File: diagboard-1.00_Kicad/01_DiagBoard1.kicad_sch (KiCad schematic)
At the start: 34 parts, among them IC1 27C512, IC2 7400N, IC3 74273N, IC4 7404N, Q1 1.000 MHz

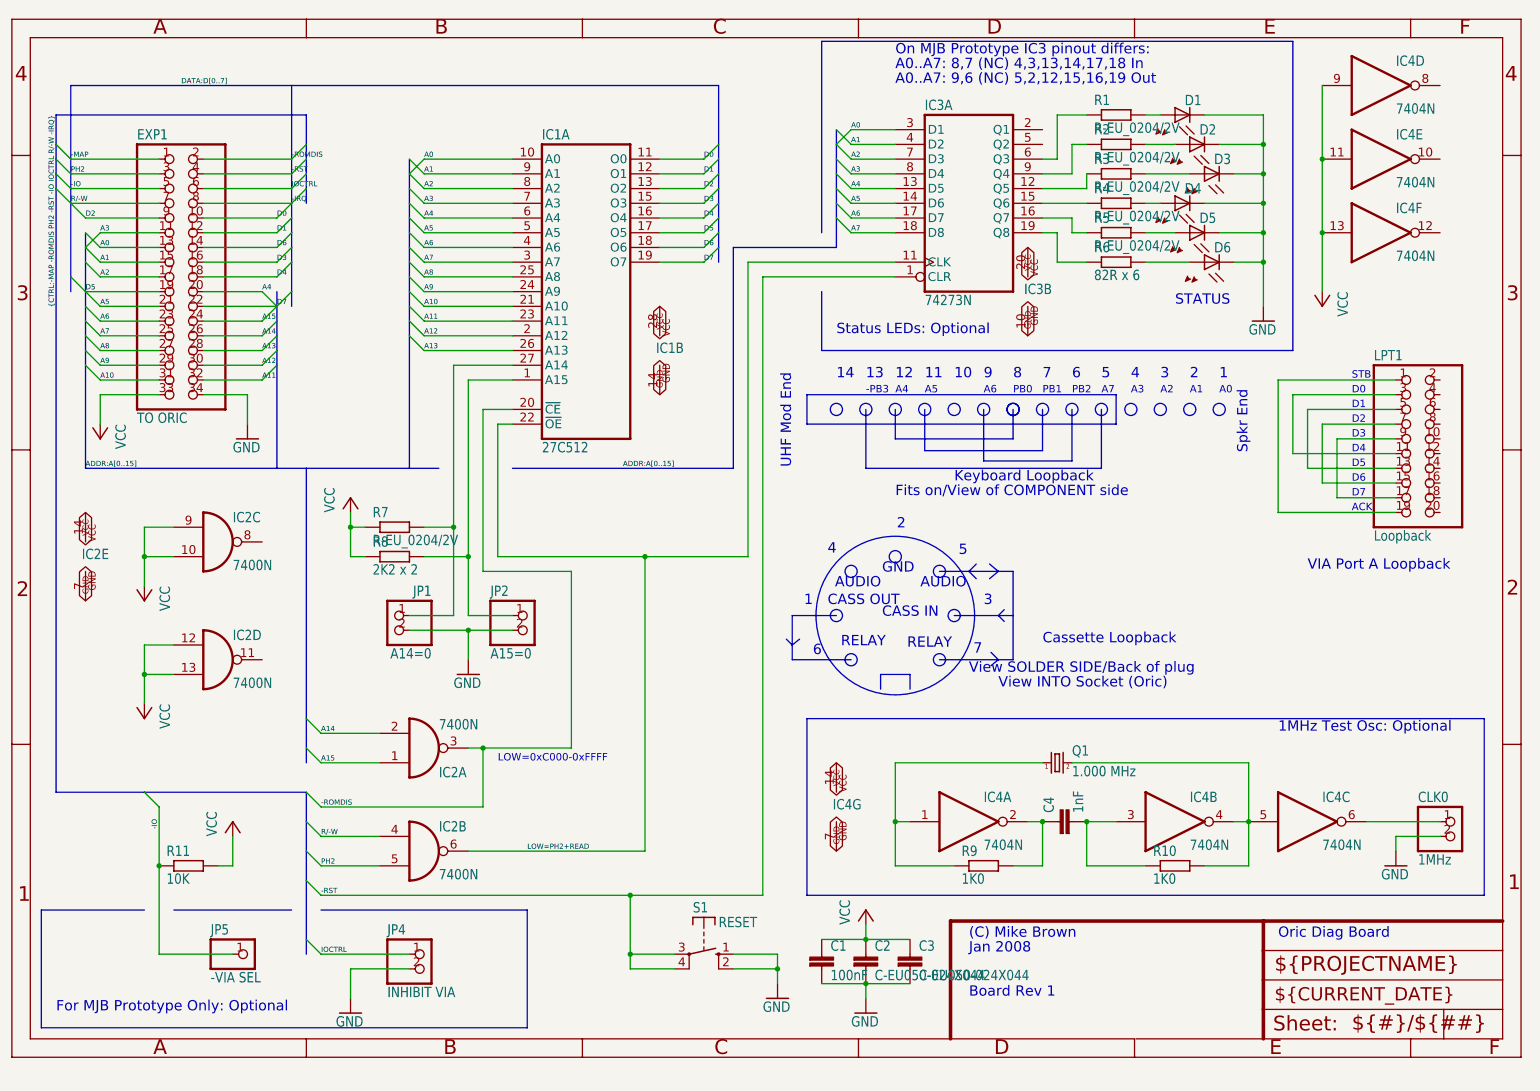
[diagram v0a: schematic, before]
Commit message: Add files via upload
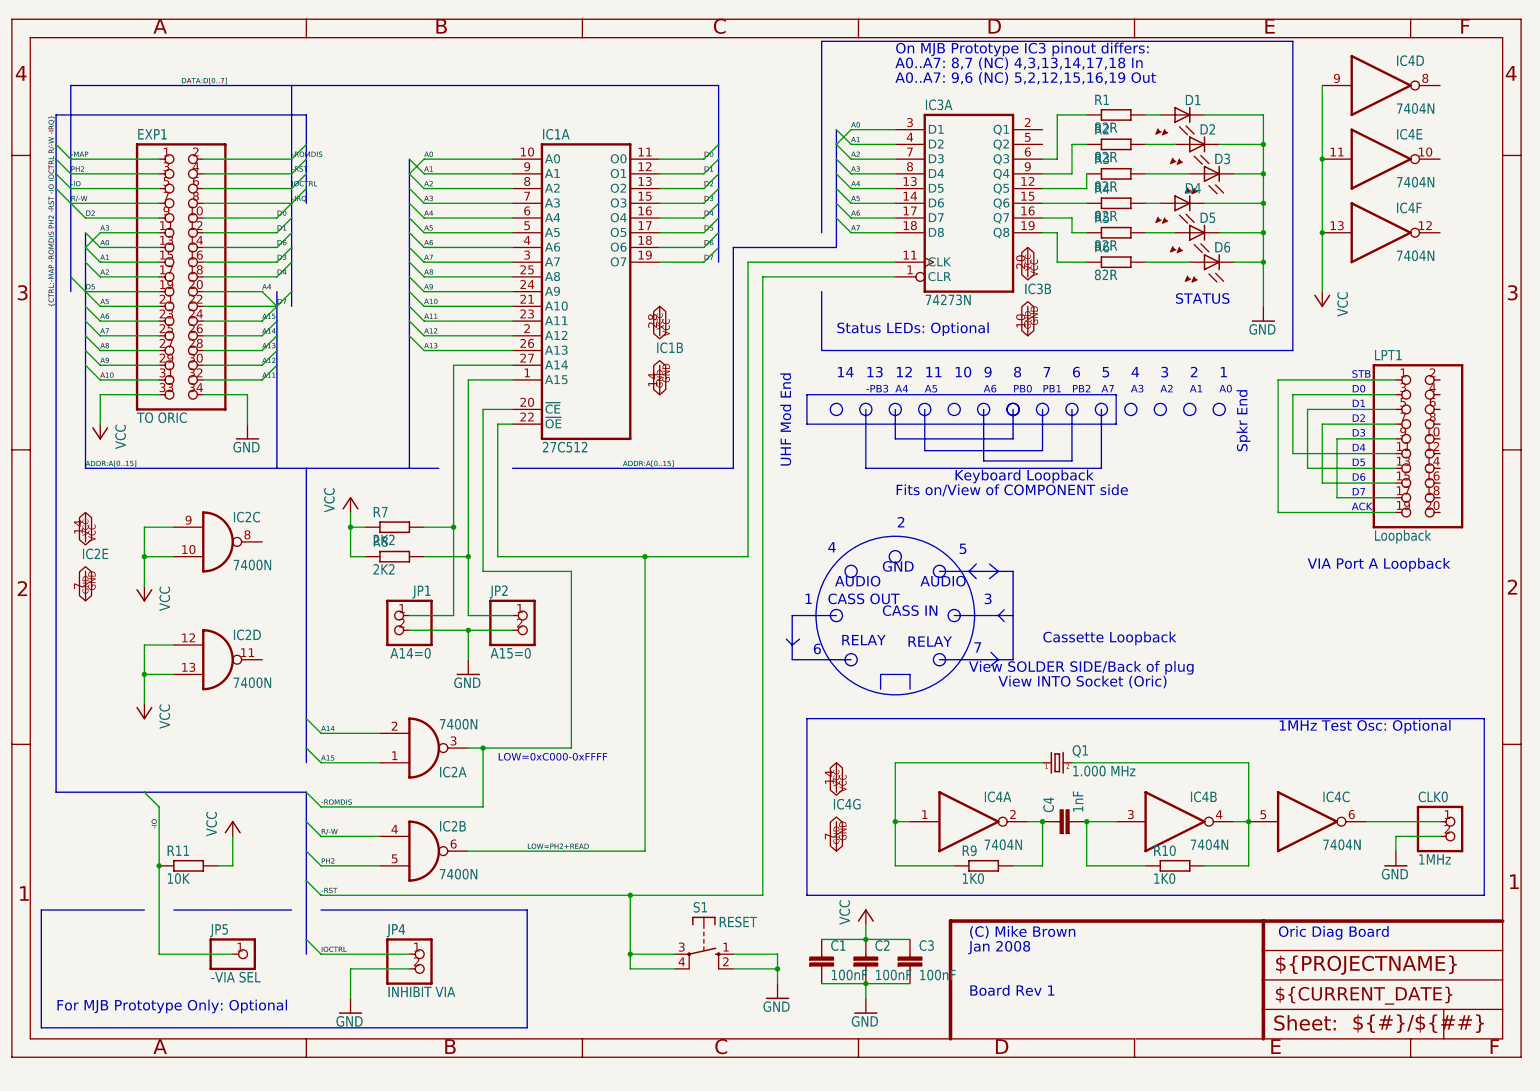
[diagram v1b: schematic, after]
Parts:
- C2, C3: value C-EU050-024X044 -> 100nF
- R1, R2, R3, R4, R5: value R-EU_0204/2V -> 82R
- R6: value 82R x 6 -> 82R
- R7: value R-EU_0204/2V -> 2K2
- R8: value 2K2 x 2 -> 2K2
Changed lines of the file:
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@@
 			)
 		)
-		(property "Value" "2K2 x 2"
+		(property "Value" "2K2"
 			(at 80.01 115.062 0)
 			(effects
@@
 			)
 		)
-		(property "Value" "C-EU050-024X044"
+		(property "Value" "100nF"
 			(at 166.624 185.039 0)
 			(effects
@@
 			)
 		)
-		(property "Value" "R-EU_0204/2V"
+		(property "Value" "82R"
 			(at 204.47 49.022 0)
 			(effects
@@
 			)
 		)
-		(property "Value" "82R x 6"
+		(property "Value" "82R"
 			(at 204.47 64.262 0)
 			(effects
@@
 			)
 		)
-		(property "Value" "R-EU_0204/2V"
+		(property "Value" "82R"
 			(at 204.47 43.942 0)
 			(effects
@@
 			)
 		)
-		(property "Value" "R-EU_0204/2V"
+		(property "Value" "82R"
 			(at 204.47 54.102 0)
 			(effects
@@
 			)
 		)
-		(property "Value" "R-EU_0204/2V"
+		(property "Value" "82R"
 			(at 204.47 59.182 0)
 			(effects
@@
 			)
 		)
-		(property "Value" "R-EU_0204/2V"
+		(property "Value" "2K2"
 			(at 80.01 109.982 0)
 			(effects
@@
 			)
 		)
-		(property "Value" "C-EU050-024X044"
+		(property "Value" "100nF"
 			(at 174.244 185.039 0)
 			(effects
@@
 			)
 		)
-		(property "Value" "R-EU_0204/2V"
+		(property "Value" "82R"
 			(at 204.47 38.862 0)
 			(effects

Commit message: Add files via upload
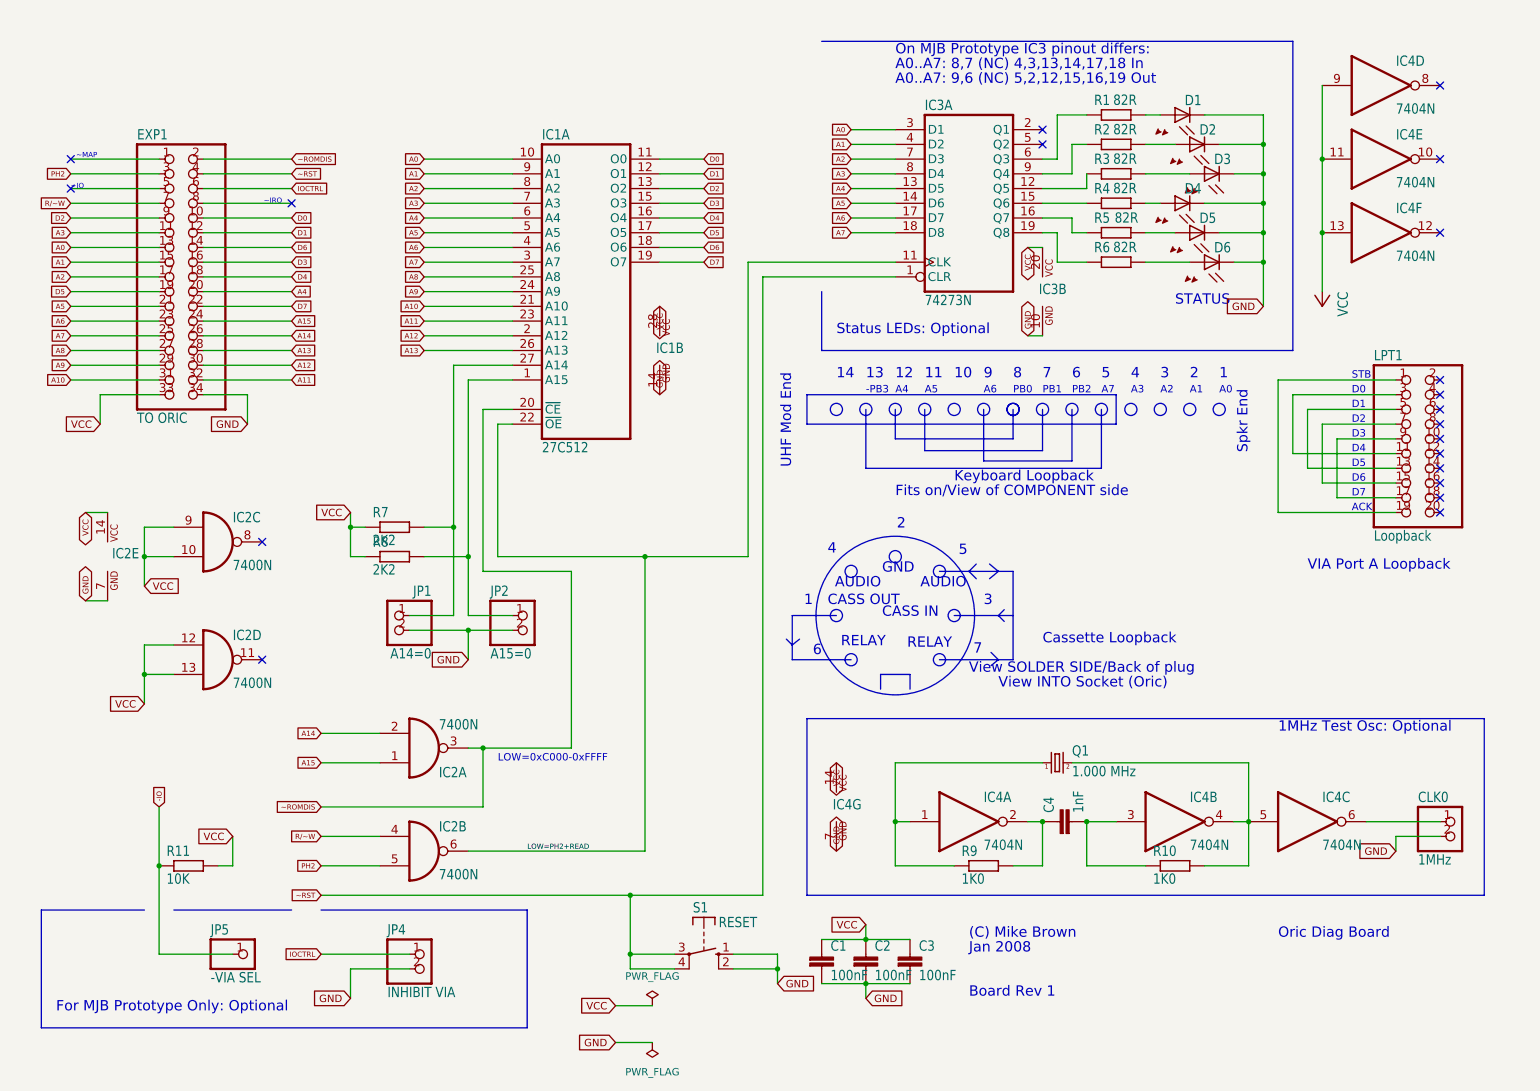
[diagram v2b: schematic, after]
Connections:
- net -IO: no longer EXP1.5
- net -IRQ: no longer names the net of EXP1.8
- net -MAP: no longer names the net of EXP1.1
- net -ROMDIS renamed ~ROMDIS
- net -RST renamed ~RST
- net R/-W renamed R/~W
- no-connect marks 0 -> 20
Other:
- note added: "~IO"
- note added: "~IRQ"
- note added: "~MAP"
- moved on the sheet: IC2E, IC3B
